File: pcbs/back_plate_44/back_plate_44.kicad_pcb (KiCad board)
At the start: 2 copper layers, 147.9 x 107.9 mm, 6 parts

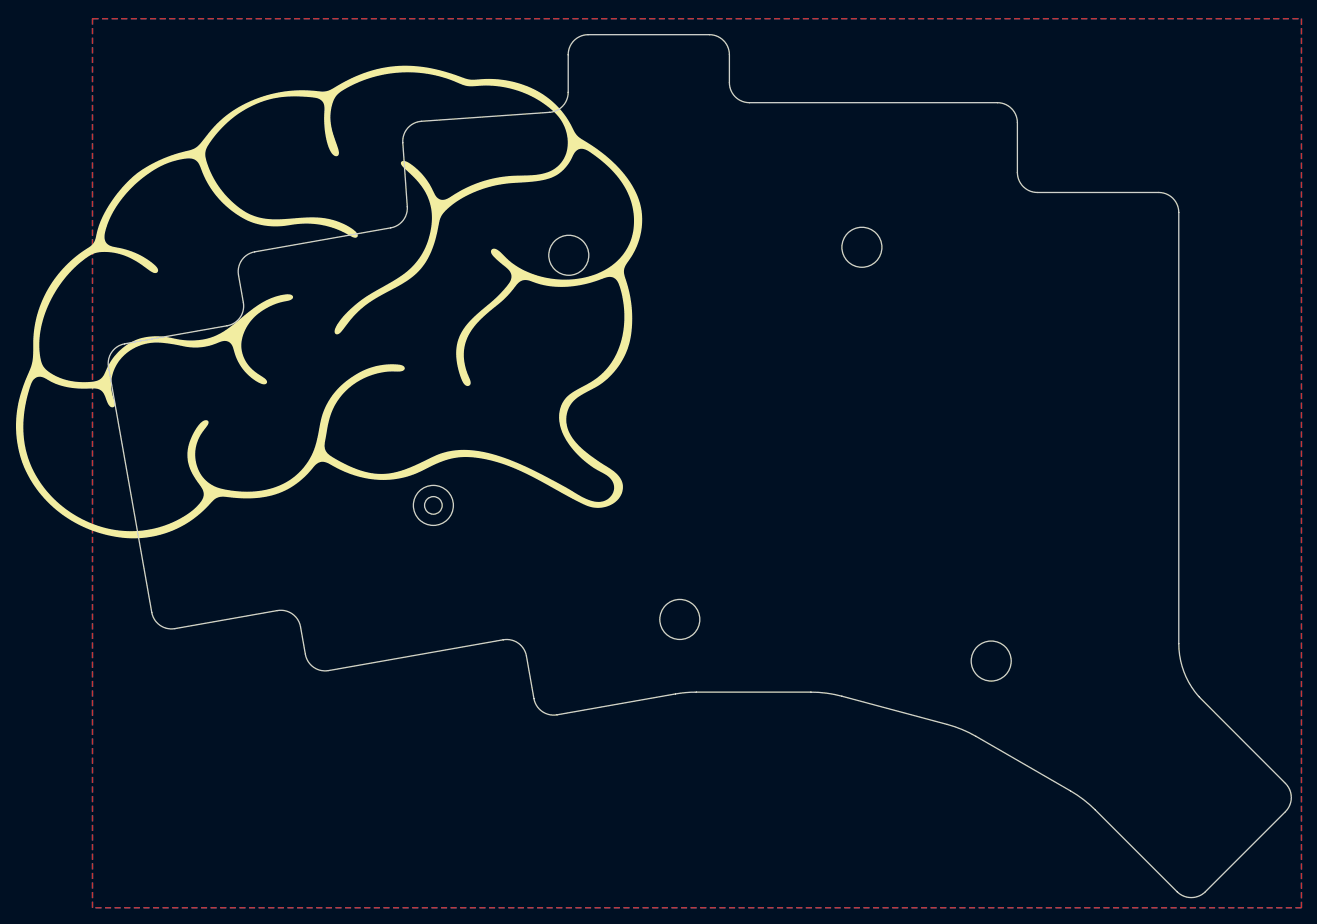
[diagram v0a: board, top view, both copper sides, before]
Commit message: update generated files
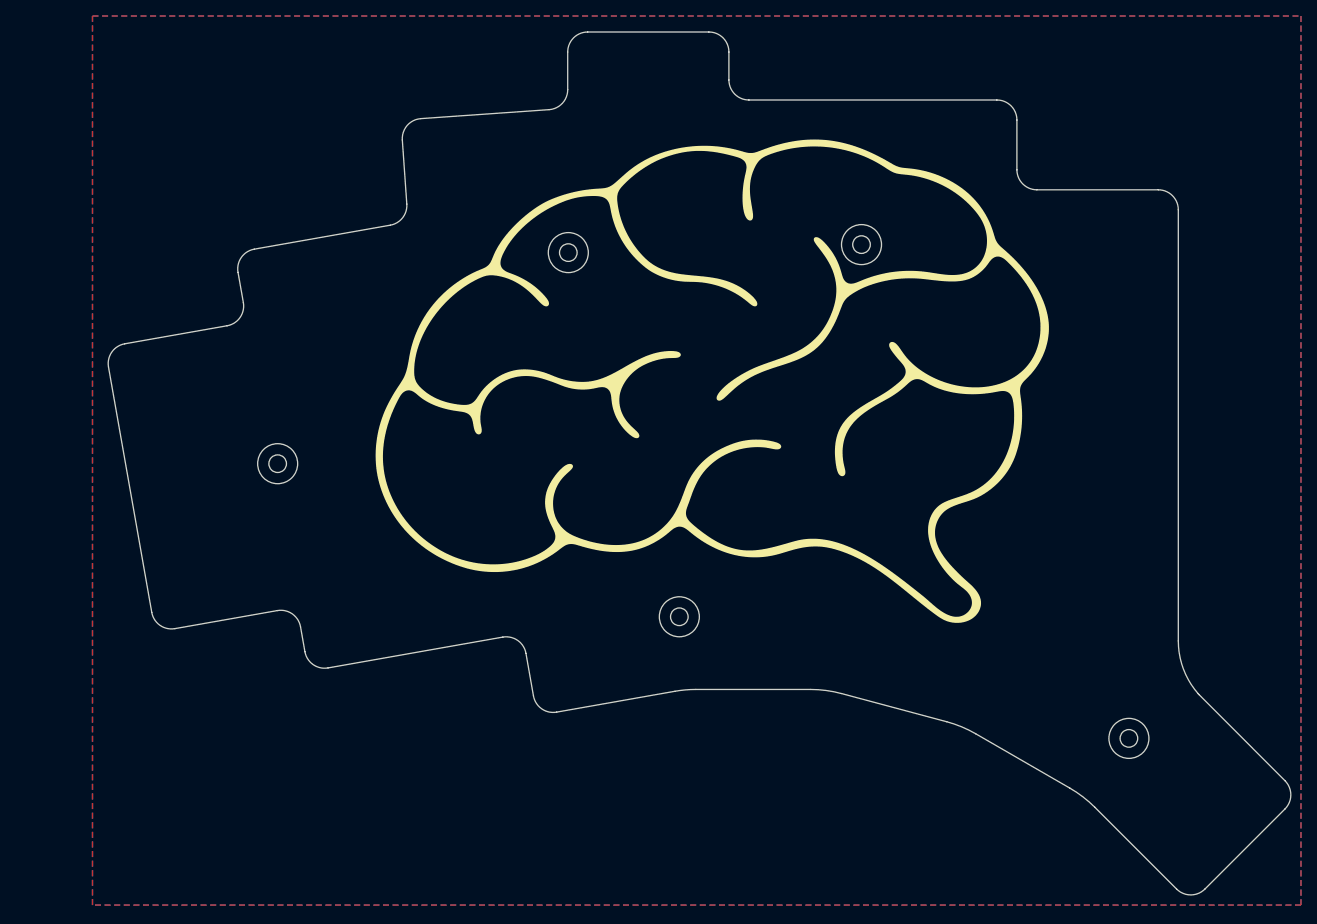
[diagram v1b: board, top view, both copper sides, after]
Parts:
- moved G1 48.7 mm to (108.4, 63.0), turned to 0 degrees
- moved MH5 20.2 mm to (54.1, 73.4), turned to 10 degrees
- moved MH3 19.7 mm to (160.5, 107.7), turned to -30 degrees
- moved MH4 0.34 mm to (104.3, 92.5)
- moved MH1 0.34 mm to (90.4, 47.0)
- moved MH2 0.34 mm to (127.1, 46.0)
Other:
- board size 147.9 x 107.9 mm -> 147.8 x 107.9 mm

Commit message: update generated files
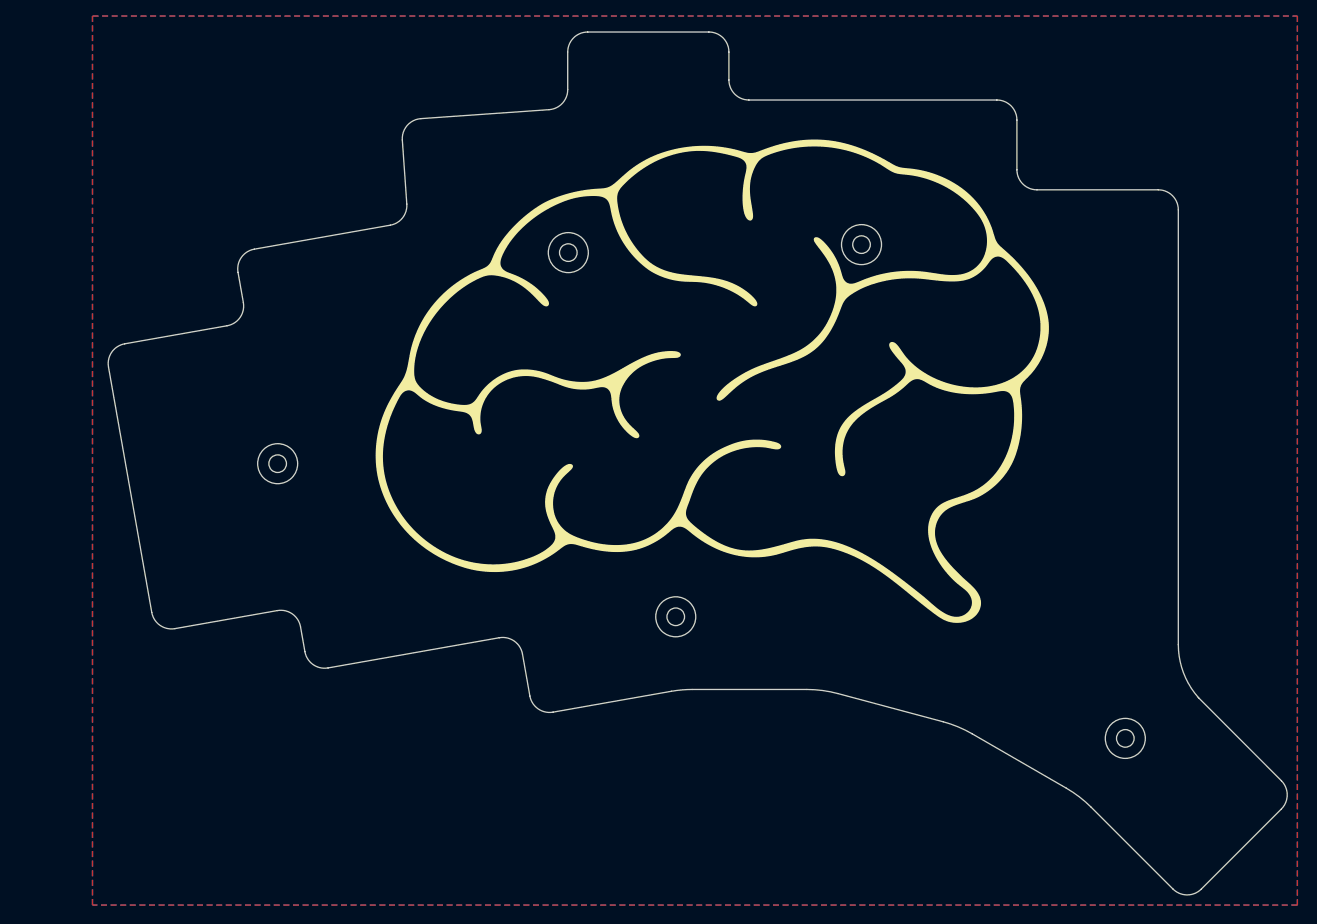
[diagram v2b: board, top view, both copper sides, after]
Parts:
- moved MH3 0.45 mm to (160.0, 107.7)
- moved MH4 0.45 mm to (103.9, 92.5)
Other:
- board size 147.8 x 107.9 mm -> 147.4 x 107.9 mm
